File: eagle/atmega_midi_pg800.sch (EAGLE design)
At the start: 19 parts, among them IC1 78L05Z, U1 6N138, U2 ATMEGA328P_PDIP, X1 MAB6H

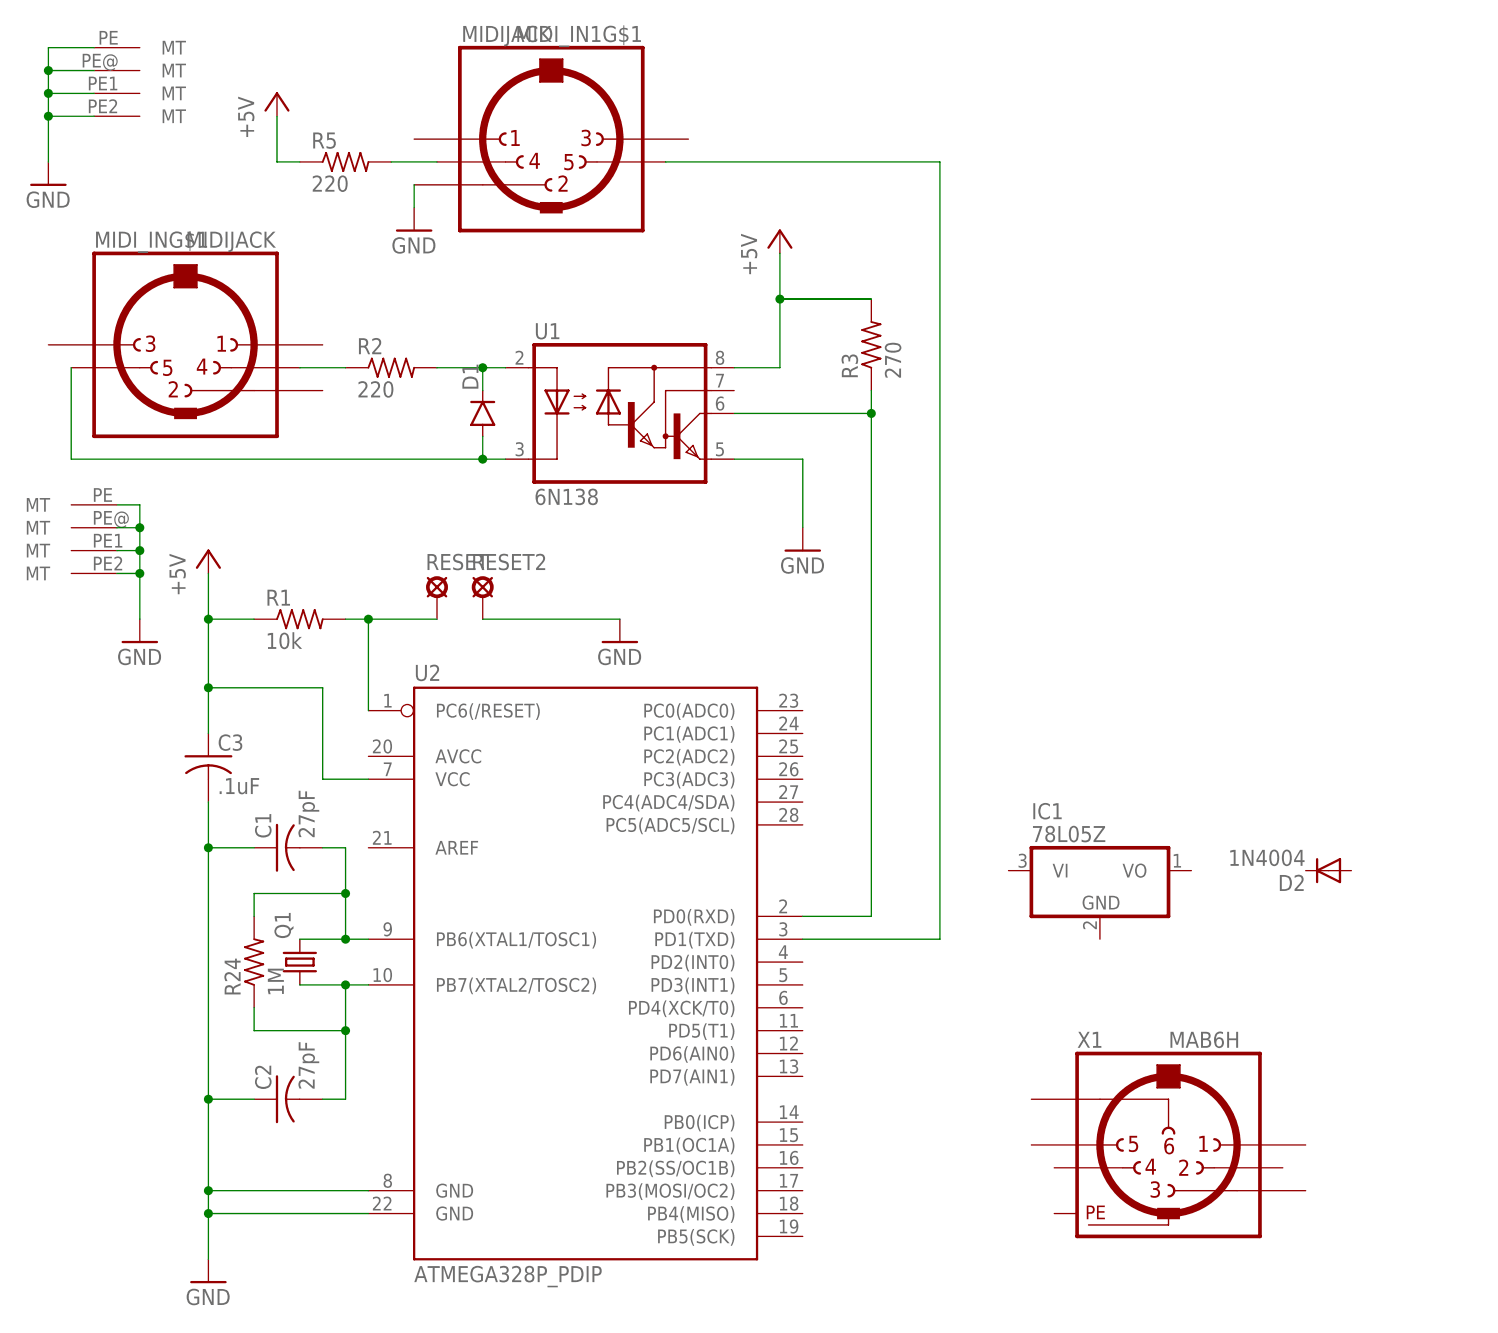
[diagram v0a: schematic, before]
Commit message: routed
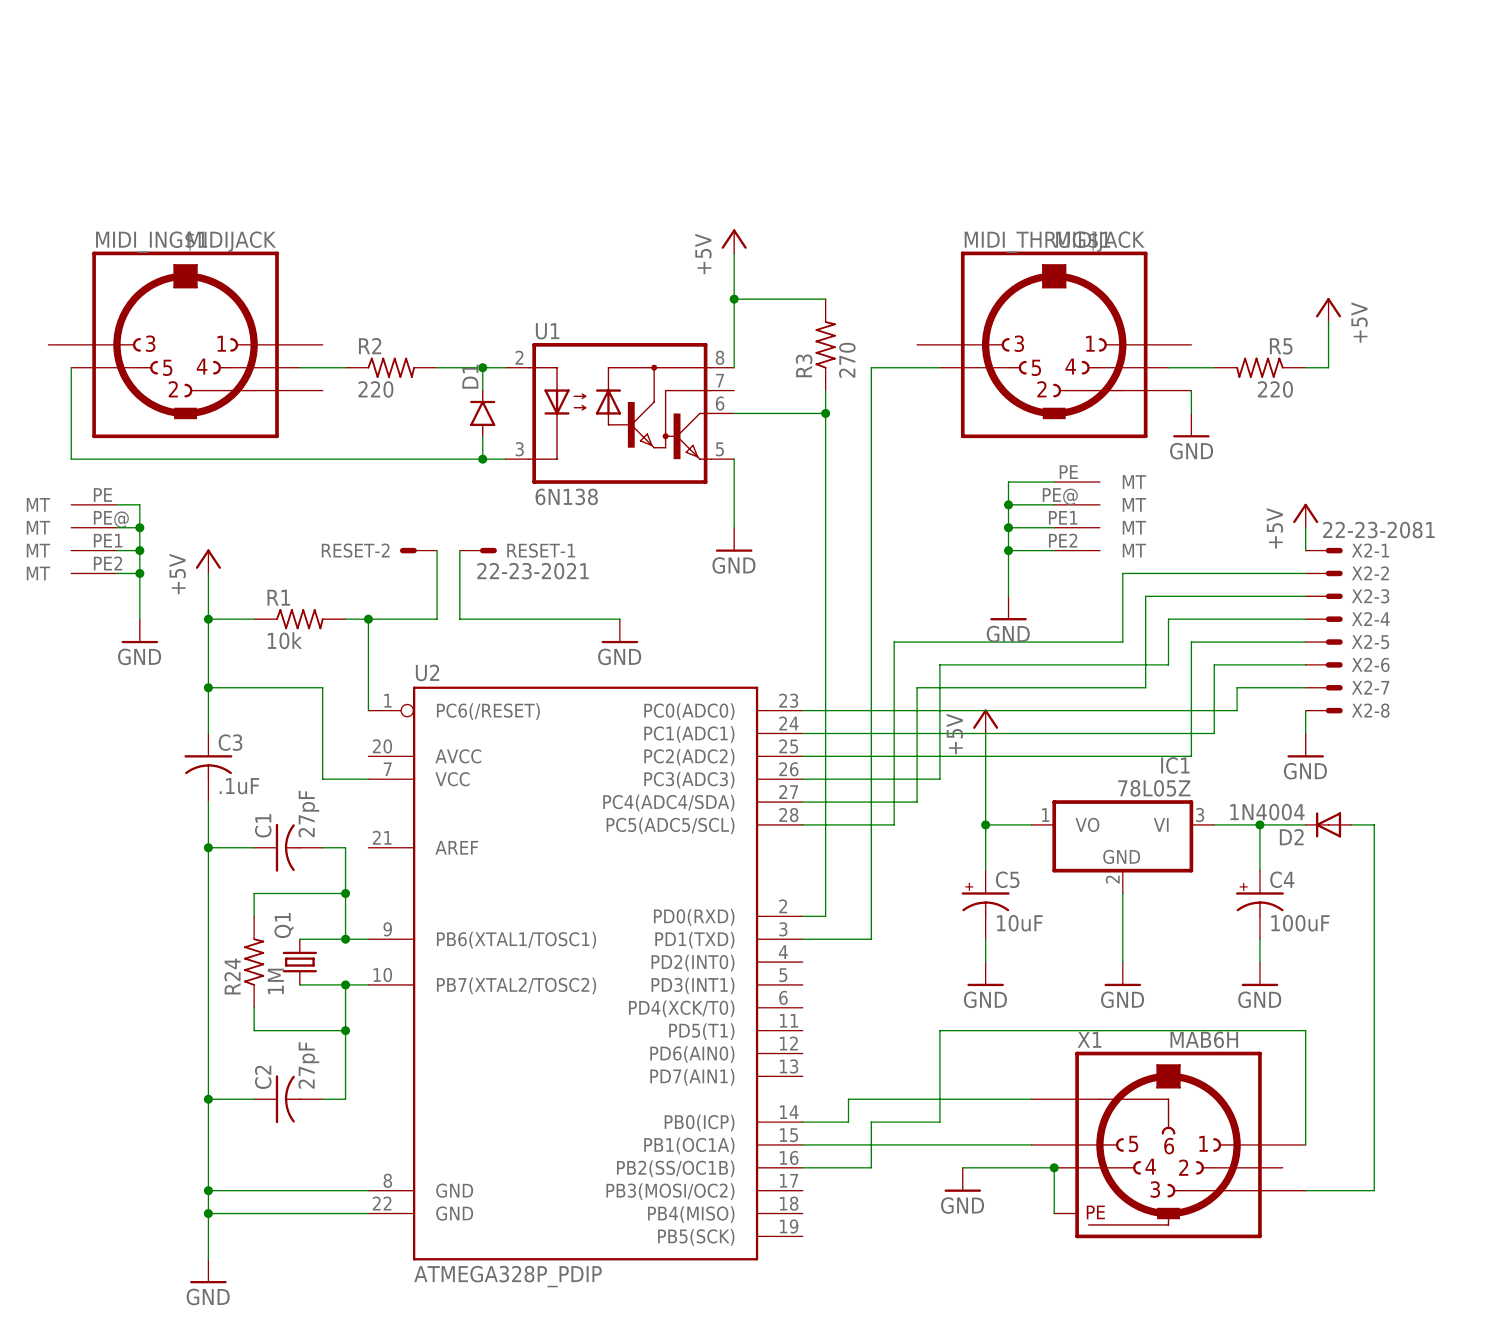
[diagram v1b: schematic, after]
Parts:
- removed MIDI_IN1: MIDIJACK, adafruit:MIDIJACK
- removed RESET2: LSP11, solpad:LSP11
- added C4: 100uF, rcl:CPOL-USB45181A
- added C5: 10uF, rcl:CPOL-USB45181A
- added MIDI_THRU: MIDIJACK, adafruit:MIDIJACK
- added X2: 22-23-2081, con-molex:22-23-2081
- RESET: value LSP11 -> 22-23-2021; device solpad:LSP11 -> con-molex:22-23-2021
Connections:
- new net N$10: U2.PB2(SS/OC1B), X1.1
- new net N$11: U2.PB1(OC1A), X1.5
- new net N$12: U2.PC0(ADC0), X2-7.S
- new net N$13: U2.PC1(ADC1), X2-6.S
- new net N$14: U2.PC2(ADC2), X2-5.S
- new net N$15: U2.PC3(ADC3), X2-4.S
- new net N$16: U2.PC4(ADC4/SDA), X2-3.S
- new net N$17: U2.PC5(ADC5/SCL), X2-2.S
- new net N$2: D2.A, X1.3
- new net N$6: C4.+, D2.C, IC1.VI
- new net N$9: U2.PB0(ICP), X1.6
- net +5V: now also C5.+, IC1.VO, X2-1.S
- net GND: now also C4.-, C5.-, IC1.GND, MIDI_THRUG$1.2, MIDI_THRUG$2.MT, MIDI_THRUG$3.MT, MIDI_THRUG$4.MT, MIDI_THRUG$5.MT, RESET-1.S, X1.4, X1.PE, X2-8.S; no longer MIDI_IN1G$1.2, MIDI_IN1G$2.MT, MIDI_IN1G$3.MT, MIDI_IN1G$4.MT, MIDI_IN1G$5.MT, RESET2.MP
- net N$1: now also MIDI_THRUG$1.4; no longer MIDI_IN1G$1.4
- net N$42: now also MIDI_THRUG$1.5; no longer MIDI_IN1G$1.5
- net N$43: now also RESET-2.S; no longer RESET.MP
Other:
- moved on the sheet: D2, IC1, R3, R5
